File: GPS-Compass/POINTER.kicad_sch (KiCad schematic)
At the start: 9 parts, among them M1 Stepper_Motor_bipolar, Q3 Q_NMOS_Depletion_GDS, U4 DRV8834PWP

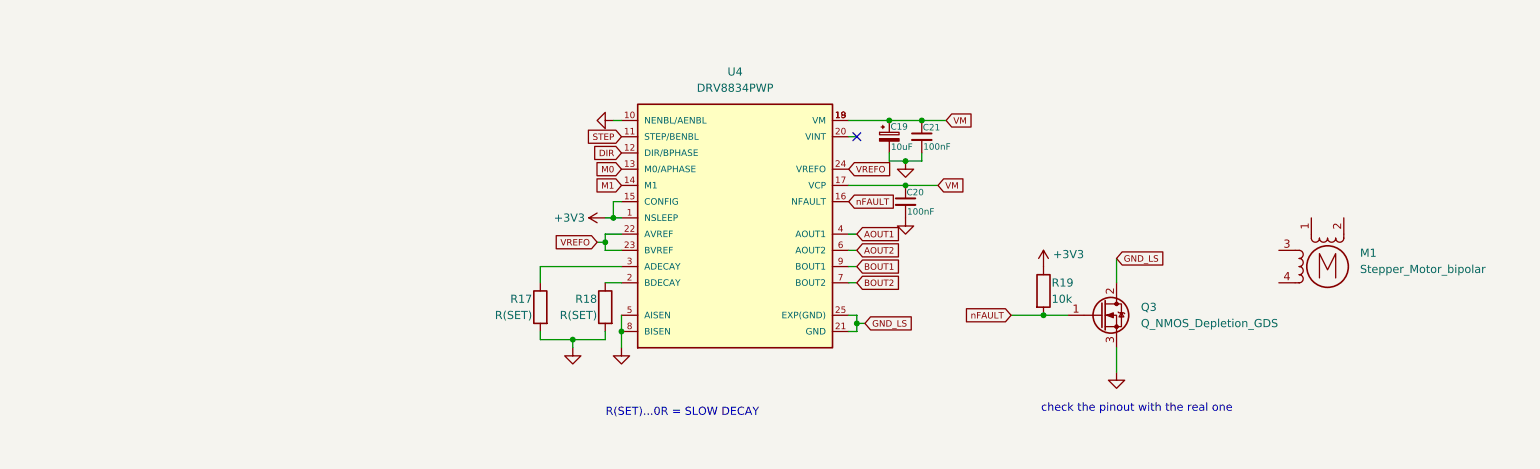
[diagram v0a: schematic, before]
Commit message: gps upd
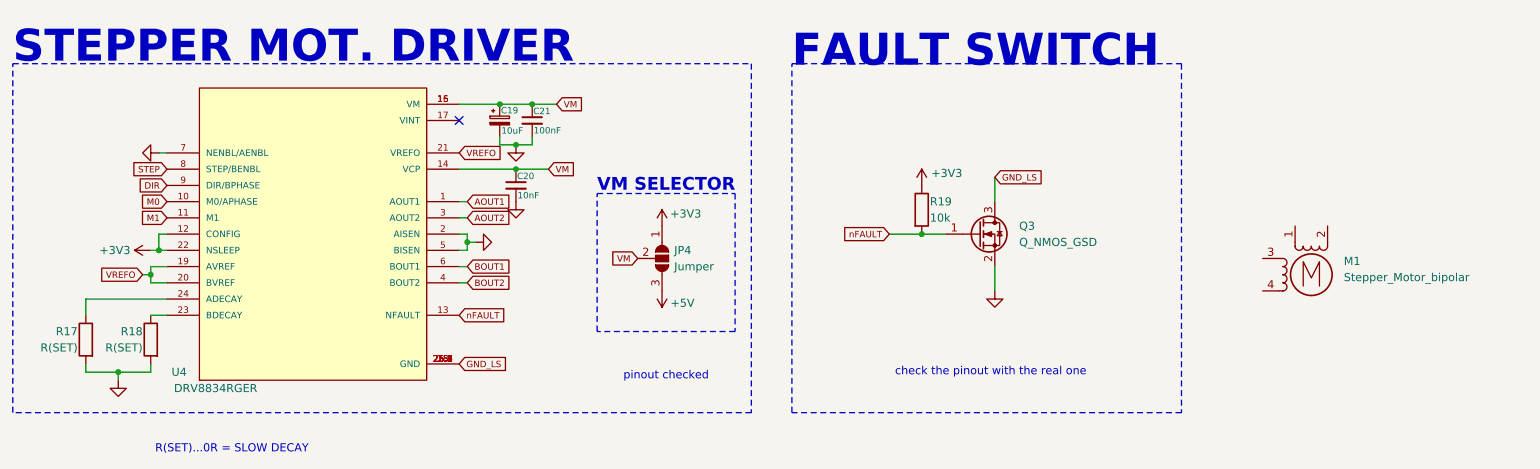
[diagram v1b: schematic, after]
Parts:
- removed Q3: Q_NMOS_Depletion_GDS, symbol Transistor_FET_Other:Q_NMOS_Depletion_GDS
- removed U4: DRV8834PWP, DRV8834PWP:SOP65P640X120-25N, symbol gps-compass_sch:DRV8834PWP
- added JP4: Jumper, Jumper:SolderJumper-3_P1.3mm_Open_RoundedPad1.0x1.5mm_NumberLabels, symbol Jumper:SolderJumper_3_Open
- added Q3: Q_NMOS_GSD, Package_TO_SOT_SMD:SOT-23-3, symbol Transistor_FET:Q_NMOS_GSD
- added U4: DRV8834RGER, gps-compass_brd:DRIVER_DRV8834RGER, symbol gps-compass_sch:DRV8834RGER
- C19: footprint (none) -> Capacitor_Tantalum_SMD:CP_EIA-3216-18_Kemet-A_Pad1.58x1.35mm_HandSolder
- C20: value 100nF -> 10nF; footprint (none) -> Capacitor_SMD:C_0402_1005Metric
- C21: footprint (none) -> Capacitor_SMD:C_0805_2012Metric
- R17, R18: footprint (none) -> Resistor_SMD:R_0805_2012Metric
- R19: footprint Resistor_THT:R_Axial_DIN0207_L6.3mm_D2.5mm_P10.16mm_Horizontal -> Resistor_SMD:R_0805_2012Metric
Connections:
- net +3V3: now also JP4.1 (A), U4.12 (CONFIG), U4.22 (NSLEEP)
- net AOUT1: now also U4.1 (AOUT1)
- net AOUT2: now also U4.3 (AOUT2)
- net BOUT1: now also U4.6 (BOUT1)
- net BOUT2: now also U4.4 (BOUT2)
- net DIR: now also U4.9 (DIR/BPHASE)
- net GND: now also Q3.2 (S), U4.2 (AISEN), U4.5 (BISEN), U4.7 (NENBL/AENBL)
- net GND_LS: now also Q3.3 (D), U4.18 (GND), U4.25 (GND), U4.25.1 (GND), U4.25.2 (GND), U4.25.3 (GND), U4.25.4 (GND), U4.25.5 (GND)
- net M0: now also U4.10 (M0/APHASE)
- net M1: now also U4.11 (M1)
- net STEP: now also U4.8 (STEP/BENBL)
- net VM: now also JP4.2 (C), U4.14 (VCP), U4.15 (VM), U4.16 (VM)
- net VREFO: now also U4.19 (AVREF), U4.20 (BVREF), U4.21 (VREFO)
- net nFAULT: now also Q3.1 (G), U4.13 (NFAULT)
- net at R17.1: now also U4.24 (ADECAY)
- net at R18.1: now also U4.23 (BDECAY)
- new net +5V: JP4.3 (B)
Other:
- note added: "FAULT SWITCH"
- note added: "STEPPER MOT. DRIVER"
- note added: "VM SELECTOR"
- note added: "pinout checked"
- moved on the sheet: C19, C20, C21, M1, R17, R18, R19
